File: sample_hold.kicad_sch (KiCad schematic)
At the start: 40 parts, among them K21 G6K-2FY, 5V, Q201 AO3400A, Q202 AO3401A, Q203 AO3400A, Q204 AO3400A, Q205 AO3400A, Q206 AO3400A, Q207 AO3400A, U19 TCA0372, U21 OPA828DGN, U22 OPA2197D

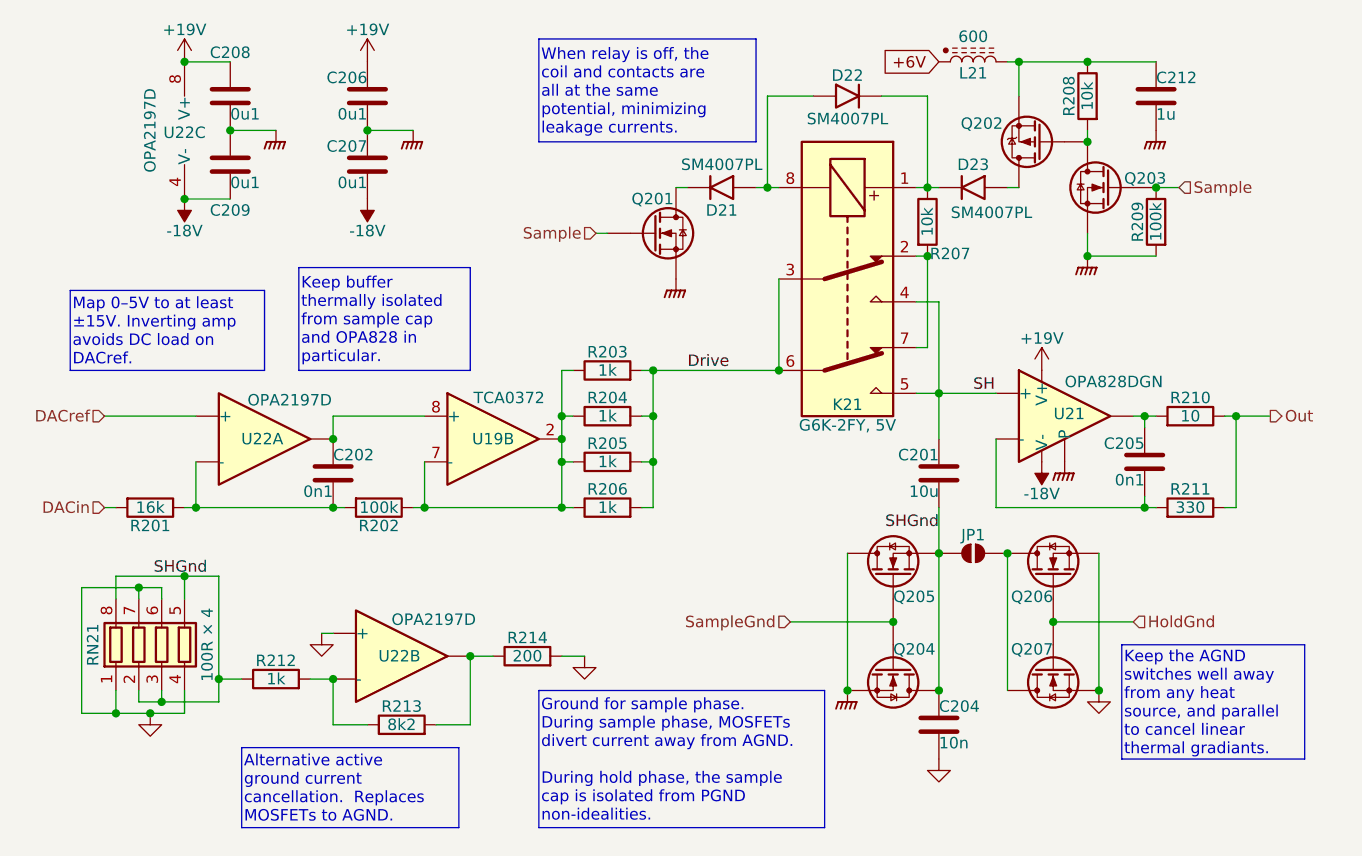
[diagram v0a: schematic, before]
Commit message: Progress checkin.  About to redo FDA feedback again.
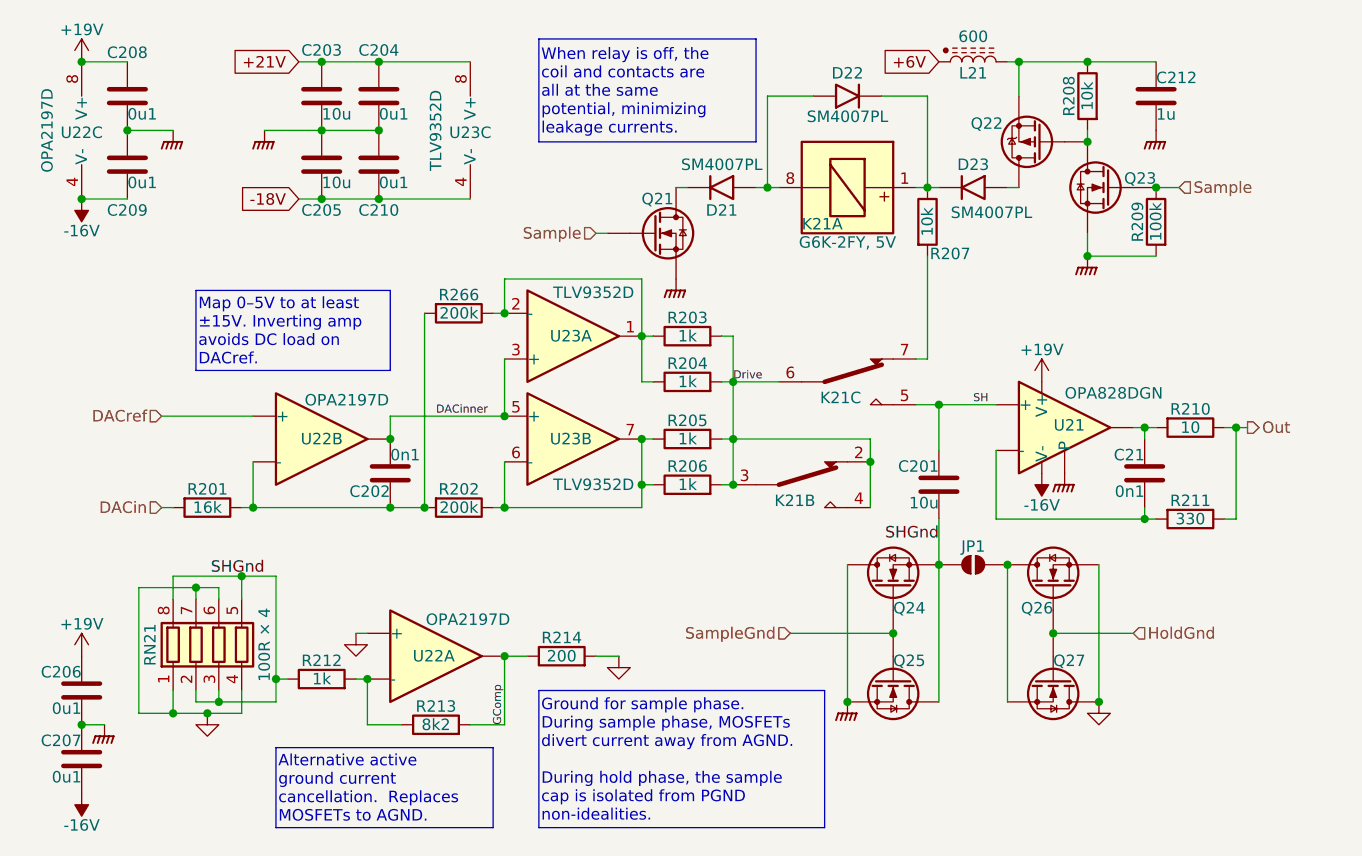
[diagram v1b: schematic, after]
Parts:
- removed U19: TCA0372, Package_SO:SOIC-16W_7.5x10.3mm_P1.27mm, symbol Parts:TCA0372
- added C203, C205: 10u, Capacitor_SMD:C_0805_2012Metric, symbol Device:C
- added C210: 0u1, Capacitor_SMD:C_0402_1005Metric, symbol Device:C
- added unit 2 of K21
- added unit 3 of K21
- added R266: 200k, Resistor_SMD:R_0402_1005Metric, symbol Device:R
- added U23: TLV9352D, Parts:TLV9352D, symbol Parts:TLV9352D
- C201: footprint Parts:C_Rect_L31.5mm_W15.0mm_P27.50mm_MKS4 -> Parts:C_Rect_L31.5mm_W15.0mm_P27.50mm_Duo
- C204: value 10n -> 0u1; footprint Capacitor_SMD:C_0603_1608Metric -> Capacitor_SMD:C_0402_1005Metric; LCSC C307500 -> C307331
- K21: footprint Relay_SMD:Relay_DPDT_Omron_G6K-2G-Y -> Relay_SMD:Relay_DPDT_Omron_G6K-2F-Y; symbol Relay:G6K-2 -> Parts:G6K_Split
- R202: value 100k -> 200k; LCSC C25741 -> (none)
- R214: footprint Resistor_SMD:R_0402_1005Metric -> Resistor_SMD:R_0603_1608Metric; LCSC C25087 -> (none)
- U21: footprint Parts:VSSOP-8-1EP_3x3mm_P0.65mm_EP1.57x1.89mm -> Parts:OPA828DGN_guard
- renumbered C205 to C21, Q201 to Q21, Q202 to Q22, Q203 to Q23, Q205 to Q24, Q204 to Q25, Q206 to Q26, Q207 to Q27
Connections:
- net -18V: now also C205.2, C210.2, U23.4 (V-); no longer C207.2, C209.2, U21.4 (V-), U22.4 (V-)
- net DACref: now also U22.5 (+); no longer U22.3 (+)
- net Drive: now also K21.2, K21.3, K21.4, K21.6; no longer K21.3, K21.6
- net GND: now also Q27.3 (D), U22.3 (+); no longer C204.2, Q27.2 (S), U22.5 (+)
- net GNDPWR: now also C204.2, C203.2, C205.1, C210.1
- net SH: now also K21.5; no longer K21.4, K21.5
- net SHGnd: no longer C204.1
- net at R201.1, R202.2: now also C202.2, U22.6 (-), R266.2; no longer C202.1, U22.2 (-)
- net at R202.1, R205.1, R206.1: now also U23.6 (-), U23.7; no longer R203.1, R204.1
- net GComp: now reaches R213.2, R214.1
- net GComp: now also U22.1; no longer U22.7
- net at JP1.2 (B), Q26.3 (D): now also Q27.2 (S); no longer Q27.3 (D)
- net at R212.2, R213.1: now also U22.2 (-); no longer U22.6 (-)
- new net: R203.1, R204.1, R266.1, U23.1, U23.2 (-)
- new net: K21.7, R207.2
- new net +21V: C203.1, C204.1, U23.8 (V+)
- new net -16V: C207.2, C209.2, U21.4 (V-), U22.4 (V-)
- new net DACinner: C202.1, U22.7, U23.3 (+), U23.5 (+)
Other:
- moved on the sheet: C201, C202, C206, C207, C208, C209, C21, D22, JP1, Q24, Q25, Q26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
